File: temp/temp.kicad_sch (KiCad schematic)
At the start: 29 parts, among them J1 Barrel_Jack, J2 Micro_SD_Card, SW1 A, SW10 4, SW11 5, SW12 6, SW13 SW_SPST, SW2 B, SW3 C, SW4 D, SW5 E, SW6 F, SW7 1, SW8 2, SW9 3, U1 AMS1117-3.3, U2 MAX98357A

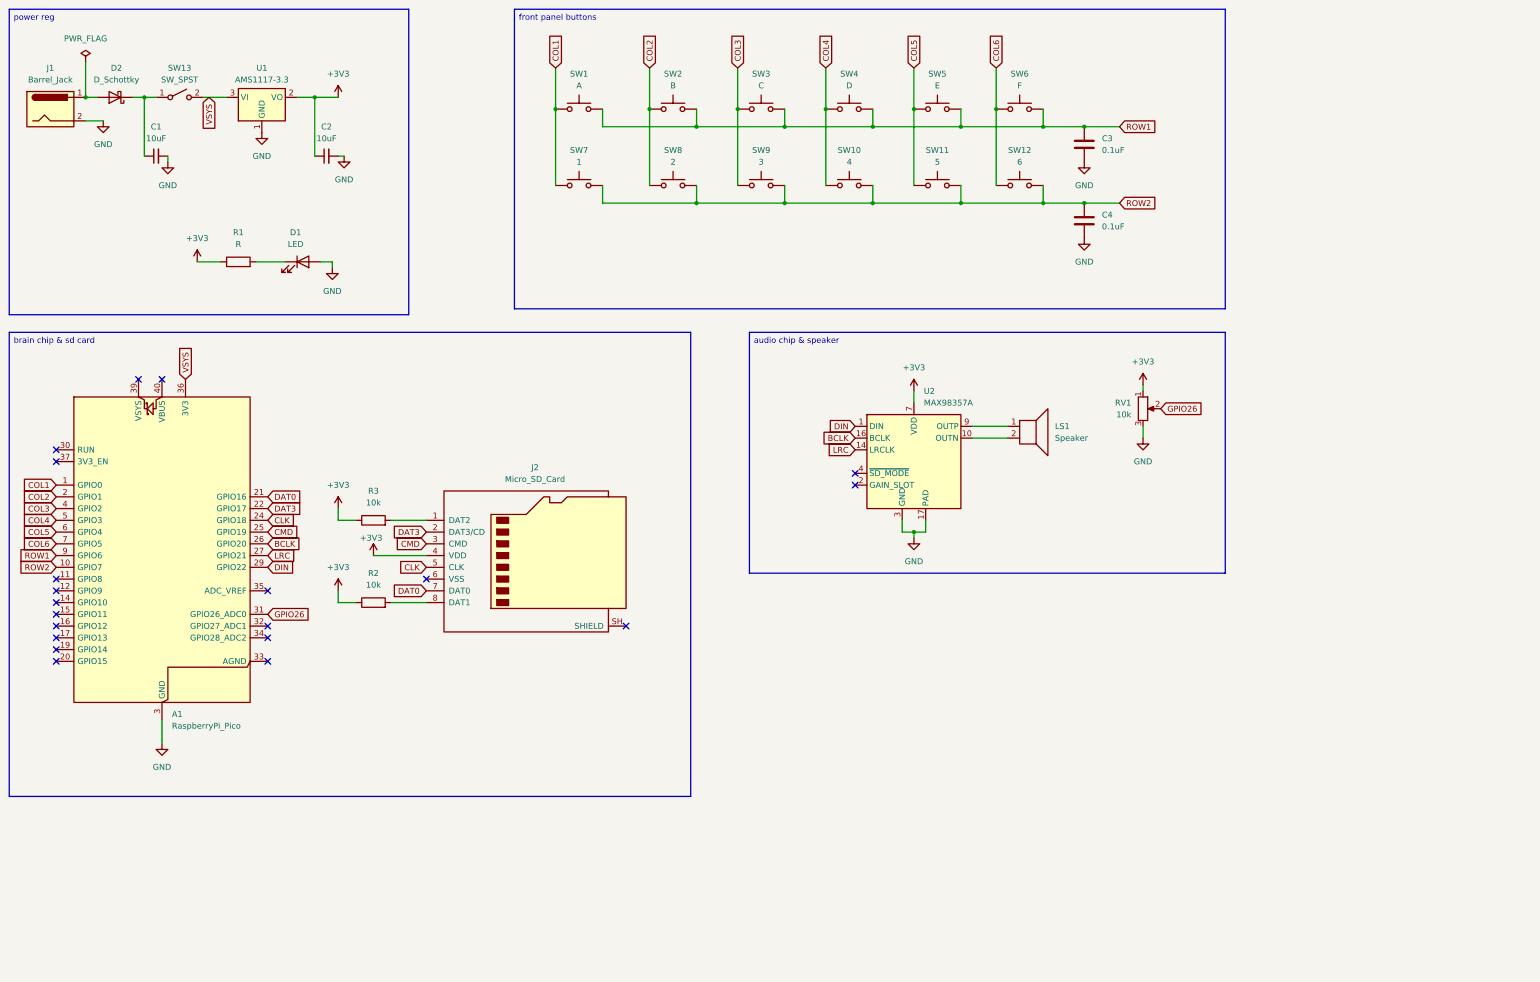
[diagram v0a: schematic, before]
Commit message: schematic review
footprints also assigned, more reviewing tomorrowww
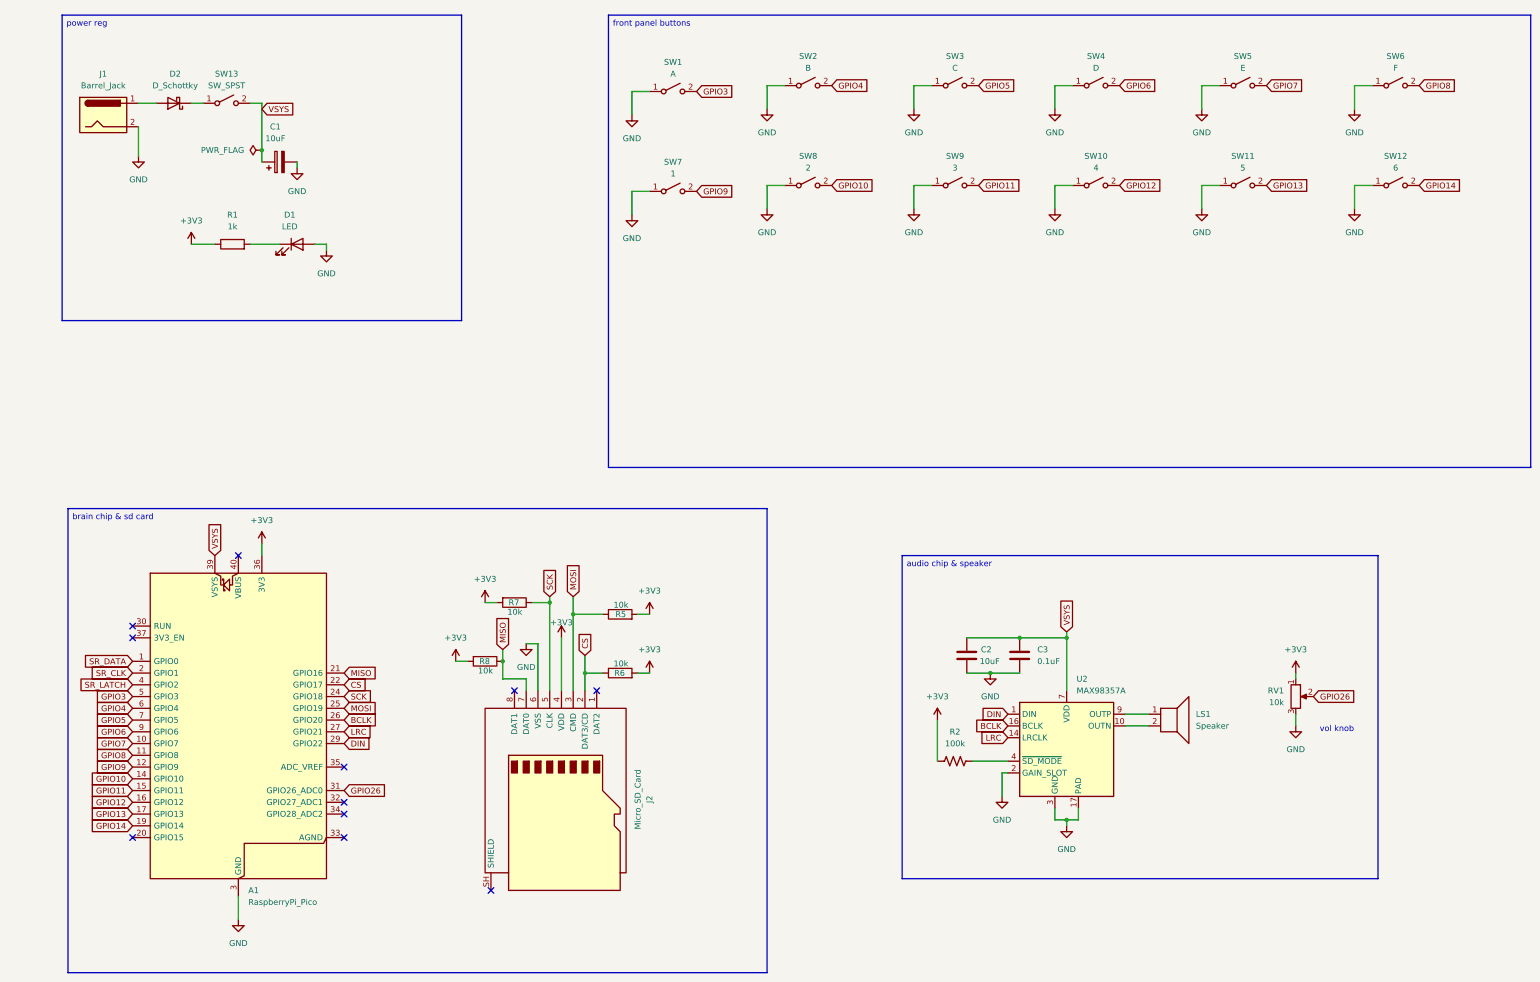
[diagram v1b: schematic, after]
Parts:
- removed C1, C2: 10uF, symbol Device:C_Small
- removed C4: 0.1uF, symbol Device:C
- removed R2, R3: 10k, symbol Device:R
- removed SW1: A, symbol Switch:SW_Push
- removed SW10: 4, symbol Switch:SW_Push
- removed SW11: 5, symbol Switch:SW_Push
- removed SW12: 6, symbol Switch:SW_Push
- removed SW2: B, symbol Switch:SW_Push
- removed SW3: C, symbol Switch:SW_Push
- removed SW4: D, symbol Switch:SW_Push
- removed SW5: E, symbol Switch:SW_Push
- removed SW6: F, symbol Switch:SW_Push
- removed SW7: 1, symbol Switch:SW_Push
- removed SW8: 2, symbol Switch:SW_Push
- removed SW9: 3, symbol Switch:SW_Push
- removed U1: AMS1117-3.3, Package_TO_SOT_SMD:SOT-223-3_TabPin2, symbol Regulator_Linear:AMS1117-3.3
- added C1: 10uF, Capacitor_THT:CP_Radial_D5.0mm_P2.00mm, symbol Device:C_Polarized
- added C2: 10uF, Capacitor_THT:CP_Radial_D5.0mm_P2.00mm, symbol Device:C
- added R2: 100k, Resistor_THT:R_Axial_DIN0207_L6.3mm_D2.5mm_P2.54mm_Vertical, symbol Device:R_US
- added R5, R6, R7, R8: 10k, Resistor_THT:R_Axial_DIN0207_L6.3mm_D2.5mm_P2.54mm_Vertical, symbol Device:R
- added SW1: A, Button_Switch_THT:SW_PUSH-12mm, symbol Switch:SW_SPST
- added SW10: 4, Button_Switch_THT:SW_PUSH-12mm, symbol Switch:SW_SPST
- added SW11: 5, Button_Switch_THT:SW_PUSH-12mm, symbol Switch:SW_SPST
- added SW12: 6, Button_Switch_THT:SW_PUSH-12mm, symbol Switch:SW_SPST
- added SW2: B, Button_Switch_THT:SW_PUSH-12mm, symbol Switch:SW_SPST
- added SW3: C, Button_Switch_THT:SW_PUSH-12mm, symbol Switch:SW_SPST
- added SW4: D, Button_Switch_THT:SW_PUSH-12mm, symbol Switch:SW_SPST
- added SW5: E, Button_Switch_THT:SW_PUSH-12mm, symbol Switch:SW_SPST
- added SW6: F, Button_Switch_THT:SW_PUSH-12mm, symbol Switch:SW_SPST
- added SW7: 1, Button_Switch_THT:SW_PUSH-12mm, symbol Switch:SW_SPST
- added SW8: 2, Button_Switch_THT:SW_PUSH-12mm, symbol Switch:SW_SPST
- added SW9: 3, Button_Switch_THT:SW_PUSH-12mm, symbol Switch:SW_SPST
- C3: footprint (none) -> Capacitor_THT:CP_Radial_D5.0mm_P2.00mm
- D1: footprint (none) -> LED_THT:LED_D10.0mm
- D2: footprint (none) -> Diode_SMD:D_3220_8050Metric_Pad2.65x5.15mm_HandSolder
- J1: footprint (none) -> Connector_BarrelJack:BarrelJack_Horizontal
- J2: footprint (none) -> Connector_Card:microSD_HC_Wuerth_693072010801
- LS1: footprint (none) -> Connector_PinHeader_2.54mm:PinHeader_1x02_P2.54mm_Vertical
- R1: value R -> 1k; footprint (none) -> Resistor_THT:R_Axial_DIN0207_L6.3mm_D2.5mm_P2.54mm_Vertical
- RV1: footprint (none) -> Potentiometer_THT:Potentiometer_Alps_RK09L_Single_Horizontal
- SW13: footprint (none) -> Button_Switch_THT:SW_Slide-03_Wuerth-WS-SLTV_10x2.5x6.4_P2.54mm
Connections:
- net +3V3: now also A1.36 (3V3), R2.1, R5.2, R6.2, R7.2, R8.2; no longer U2.7 (VDD), U2.8 (VDD)
- net GND: now also J2.6 (VSS), U2.2 (GAIN_SLOT), C1.2, C2.2, SW1.1 (A), SW10.1 (A), SW11.1 (A), SW12.1 (A), SW2.1 (A), SW3.1 (A), SW4.1 (A), SW5.1 (A), SW6.1 (A), SW7.1 (A), SW8.1 (A), SW9.1 (A)
- net VSYS: now also A1.39 (VSYS), C3.1, U2.7 (VDD), U2.8 (VDD), C1.1, C2.1; no longer A1.36 (3V3)
- net GPIO8: now reaches A1.11 (GPIO8)
- net GPIO8: now also SW6.2 (B)
- net GPIO9: now reaches A1.12 (GPIO9)
- net GPIO9: now also SW7.2 (B)
- net GPIO10: now reaches A1.14 (GPIO10)
- net GPIO10: now also SW8.2 (B)
- net GPIO11: now reaches A1.15 (GPIO11)
- net GPIO11: now also SW9.2 (B)
- net GPIO12: now reaches A1.16 (GPIO12)
- net GPIO12: now also SW10.2 (B)
- net GPIO13: now reaches A1.17 (GPIO13)
- net GPIO13: now also SW11.2 (B)
- net GPIO14: now reaches A1.19 (GPIO14)
- net GPIO14: now also SW12.2 (B)
- net at U2.4 (~{SD_MODE}): now also R2.2
- net CLK renamed SCK
- net SCK: now also R7.1
- net CMD renamed MOSI
- net MOSI: now also R5.1
- net COL1 renamed SR_DATA
- net COL2 renamed SR_CLK
- net COL3 renamed SR_LATCH
- net COL4 renamed GPIO3
- net GPIO3: now also SW1.2 (B)
- net COL5 renamed GPIO4
- net GPIO4: now also SW2.2 (B)
- net COL6 renamed GPIO5
- net GPIO5: now also SW3.2 (B)
- net DAT0 renamed MISO
- net MISO: now also R8.1
- net DAT3 renamed CS
- net CS: now also R6.1
- net ROW1 renamed GPIO6
- net GPIO6: now also SW4.2 (B); no longer C3.1
- net ROW2 renamed GPIO7
- net GPIO7: now also SW5.2 (B)
- no-connect marks 20 -> 11
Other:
- note added: "vol knob"
- moved on the sheet: A1, D1, D2, J1, J2, LS1, R1, RV1, U2
